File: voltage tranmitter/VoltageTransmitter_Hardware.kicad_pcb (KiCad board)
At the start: 2 copper layers, 11 parts, among them U1 AP1059, U2 ESP8266_MCU

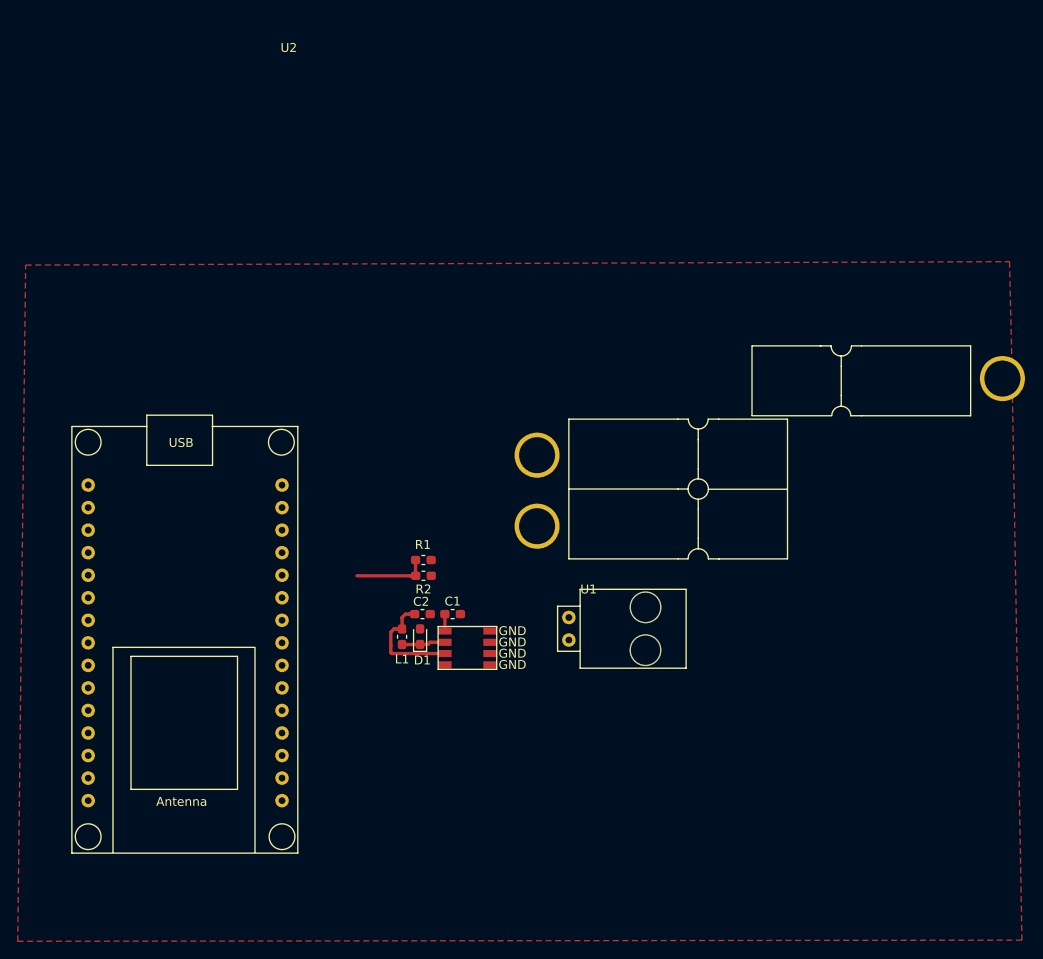
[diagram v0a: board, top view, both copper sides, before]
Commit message: Did the traces for the PCB
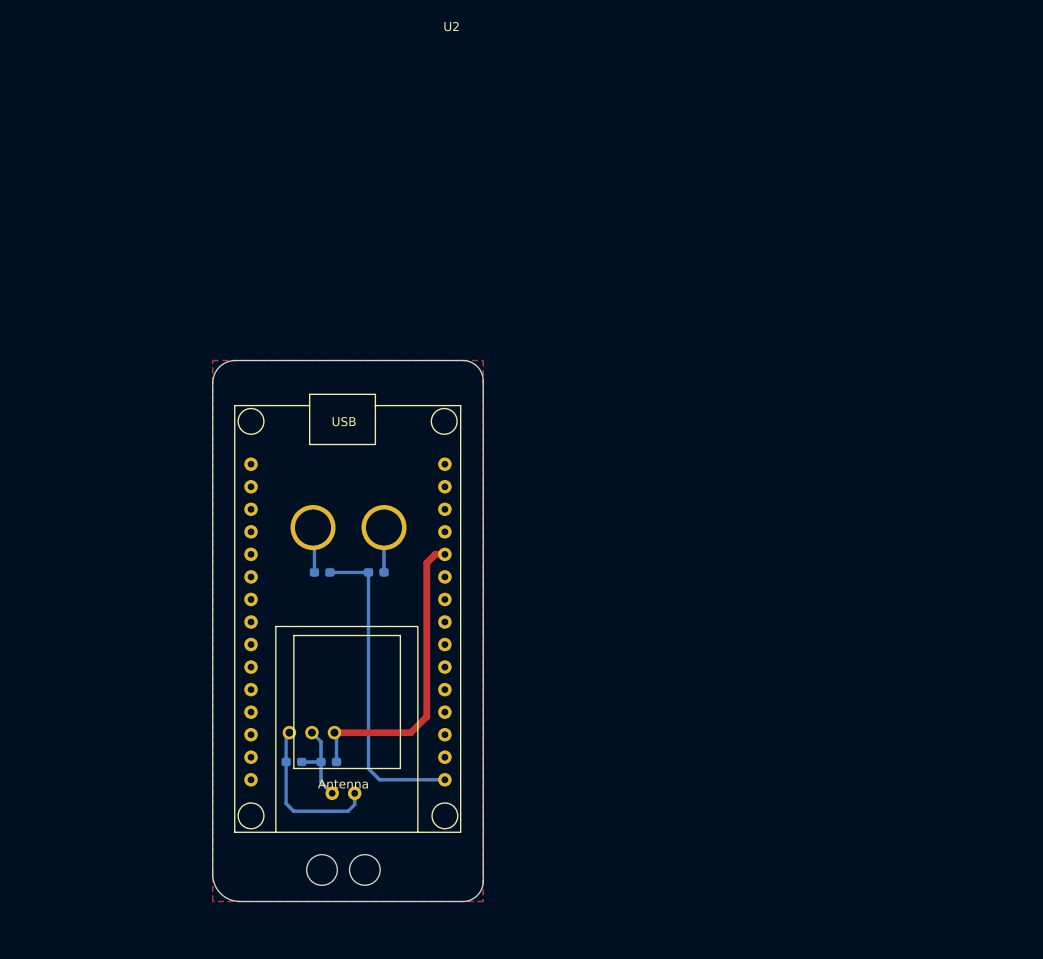
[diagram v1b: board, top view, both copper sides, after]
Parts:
- removed Conn3: AndersonPP-MRDT_Connectors, MRDT_Connectors:Anderson_1_Horisontal
- removed D1: D_Schottky, Diode_SMD:D_0603_1608Metric_Pad1.05x0.95mm_HandSolder
- removed L1: 47uH, Inductor_SMD:L_0603_1608Metric_Pad1.05x0.95mm_HandSolder
- C1, C2, Conn1, Conn2, R1, R2: moved to B.Cu
- U1: value AP1059 -> OKI; footprint MRDT_Devices:AP1509 -> MRDT_Devices:OKI_Horizontal; moved to B.Cu
- moved Conn2 31.4 mm to (131.6, 104.6), turned to 0 degrees
- moved U1 29.9 mm to (122.9, 99.1)
- moved C1 24.4 mm to (126.0, 101.1)
- moved C2 19.7 mm to (129.9, 101.1)
- moved Conn1 18.9 mm to (140.2, 71.1), turned to 270 degrees
- moved U2 18.5 mm to (144.8, 61.0)
- moved R1 11.5 mm to (129.2, 79.8), turned to 0 degrees
- moved R2 5.33 mm to (135.3, 79.8)
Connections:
- C1 pad 2: GND -> Net-(C1-Pad2)
- C2 pad 1: GND -> +3V3
- C2 pad 2: +3V3 -> Net-(C1-Pad2)
- Conn2 pad 1: Net-(C1-Pad1) -> Net-(C1-Pad2)
- Conn2 pad 2: GND -> Net-(C1-Pad1)
- U1 pad 2: Net-(D1-Pad1) -> Net-(C1-Pad2)
- U2 pad 1: Net-(U2-Pad1) -> Din
- U2 pad 12: Din -> Net-(U2-Pad12)
- U2 pad 24: Net-(U2-Pad24) -> GND
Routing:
- net Din: track 8.38 -> 35.6 mm
- net +3V3: track 12.7 -> 34.3 mm
- net Net-(C1-Pad1): track 1.65 -> 17.8 mm
- net Net-(C1-Pad2): track 0.00 -> 9.96 mm
- net Net-(D1-Pad1): track 5.18 -> 0.00 mm
- net Net-(Conn1-Pad2): track 0.00 -> 5.12 mm
- net GND: track 0.00 -> 5.06 mm
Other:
- board outline added: 30.5 x 61 mm
